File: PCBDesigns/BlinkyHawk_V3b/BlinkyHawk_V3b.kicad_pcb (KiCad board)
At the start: 4 copper layers, 25.4 x 55 mm, 41 parts, among them J1 Conn_01x01, J2 Conn_01x01, J3 Conn_01x07_Pin, J4 Battery, J5 Conn_01x01, J6 Conn_01x07_Pin, J7 Conn_01x01, Q1 AO3400A MOSFET, U1 TPS22914BYFPR, U3 TL431DBZ, U4 TPS22914BYFPR, U5 PAM8904JER

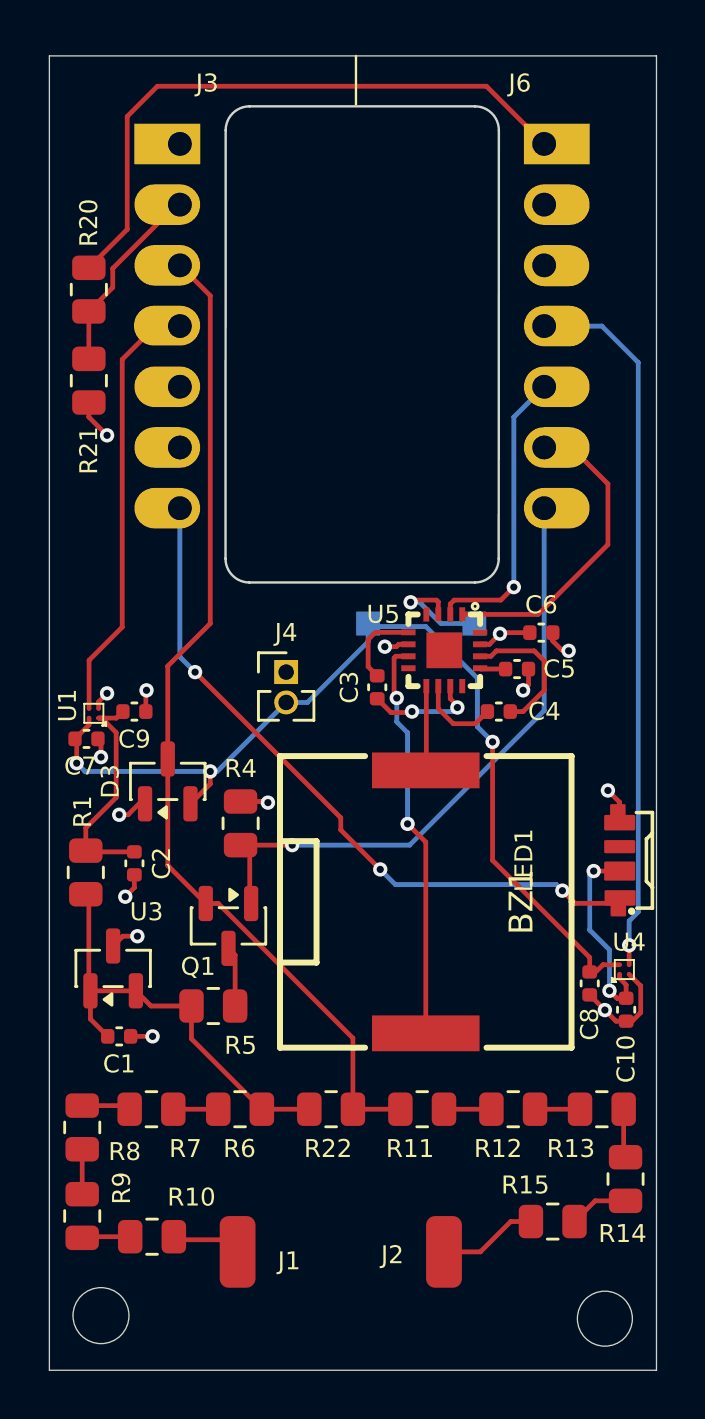
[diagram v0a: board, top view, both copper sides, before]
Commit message: AD8237DevBoardTestDesign
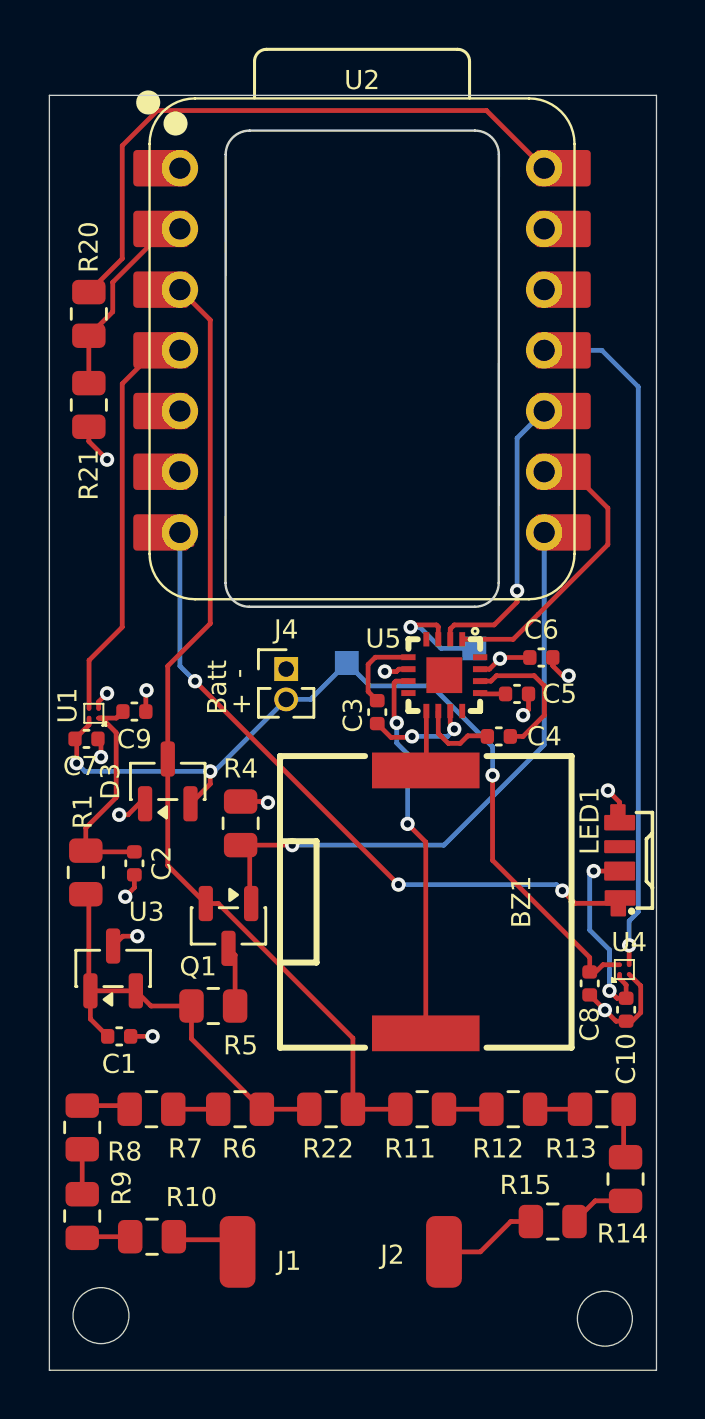
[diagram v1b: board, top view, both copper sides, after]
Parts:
- removed J3, J6: Conn_01x07_Pin, Connector_PinSocket_2.54mm:PinSocket_1x07_P2.54mm_Vertical
- added U2: ~, Seeed_XIAO:XIAO-R4-DIP, F.Cu at (158.6, 73.3)
- C2: value 0.47uF -> 1uF
- moved J5 1.88 mm to (158.0, 86.4)
- moved C4 1.04 mm to (164.3, 89.4)
- moved C3 1.04 mm to (159.3, 88.4)
- moved C5 1.04 mm to (165.1, 87.7)
- moved C6 1.04 mm to (166.1, 86.1)
- moved J7 1.04 mm to (163.3, 85.7)
- moved U5 1.04 mm to (162.1, 86.9)
- moved R20 1.02 mm to (147.2, 71.8)
- moved R21 1.02 mm to (147.2, 75.6)
- moved J4 0.13 mm to (155.4, 86.6)
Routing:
- net BatteryRail: track 40.0 -> 37.0 mm
- net D6: track 29.9 -> 28.8 mm
- net Net-(BZ1--): track 16.9 -> 15.8 mm
- net A3: track 19.0 -> 18.0 mm
- net A2: track 42.1 -> 41.1 mm
- net D10: track 29.9 -> 28.9 mm
- net Net-(BZ1-+): track 3.19 -> 2.50 mm
- net D8: track 13.1 -> 12.6 mm
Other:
- board size 25.4 x 55 mm -> 25.4 x 53.3 mm
- board text added: "OIH Designs {dblquote}Blinky Hawk{dblquote} 20260916"
- board text removed: "OIH Designs {dblquote}Blinky Hawk{dblquote} 20260801"
